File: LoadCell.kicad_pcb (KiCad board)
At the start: 2 copper layers, 51.1 x 38.1 mm, 83 parts, among them J1 M20-8760242, J10 M20-8760242, J11 0.100_1X4, J12 0.100_1X4, J13 M20-8760242, J14 M20-8760242, J15 0.100_1X4, J16 0.100_1X4, J2 M20-8760242, J3 0.100_1X4, J4 0.100_1X4, J5 M20-8760242, J6 M20-8760242, J7 0.100_1X4, J8 0.100_1X4, J9 M20-8760242, U1 MCP6002, U2 MCP6002, U3 MCP6002, U4 MCP6002, U5 MCP6002, U6 MCP6002, U7 MCP6002, U8 MCP6002

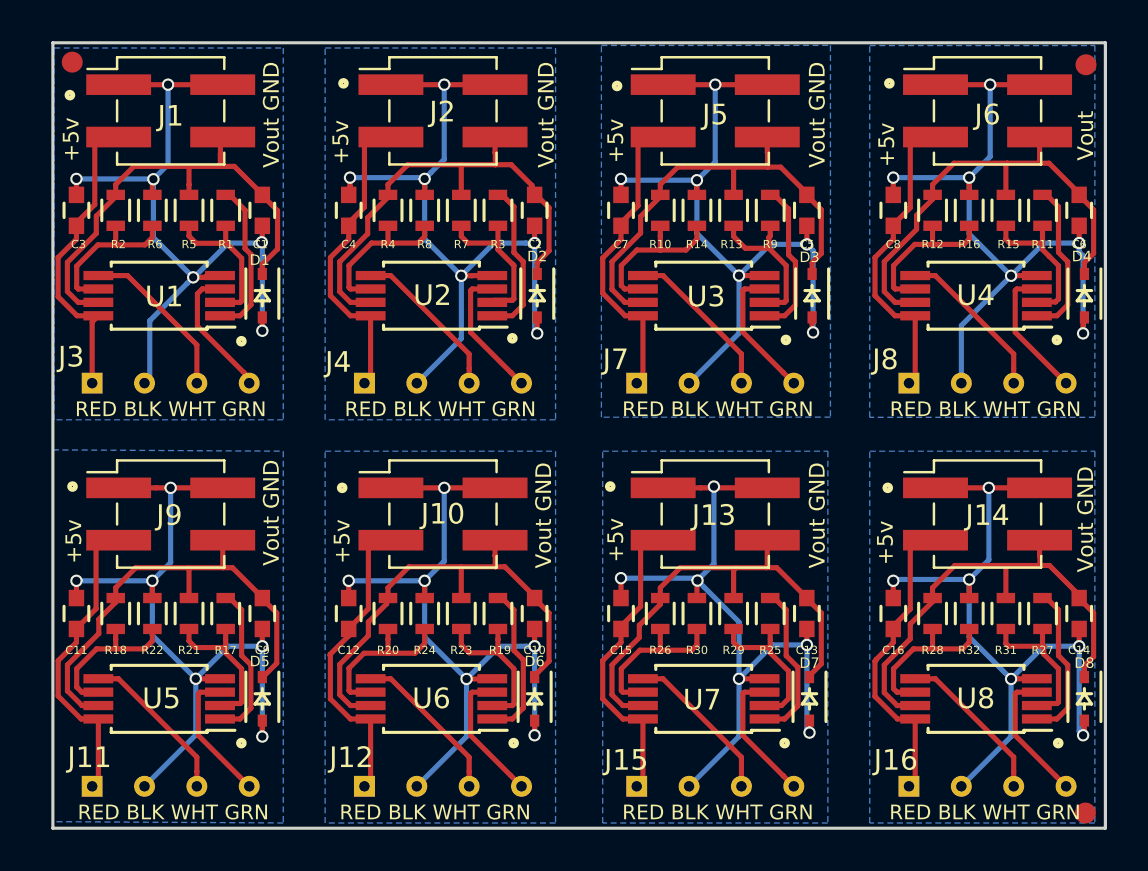
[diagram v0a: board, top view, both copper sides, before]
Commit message: First cut
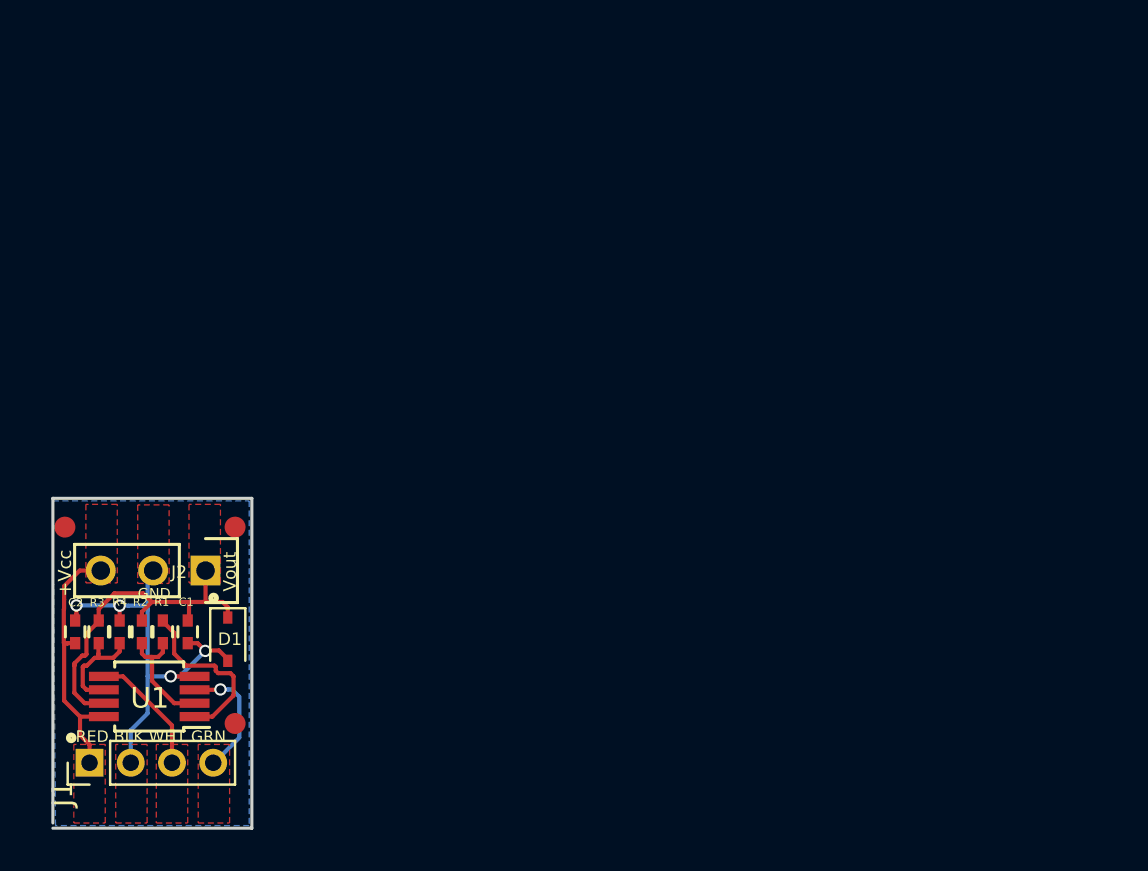
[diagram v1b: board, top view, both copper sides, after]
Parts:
- removed C10, C11, C12, C13, C14, C15, C16, C3, C4, C5, C6, C7, C8, C9: 1uF, _Passive:C_0603
- removed D2, D3, D4, D5, D6, D7, D8: MM3Z3V0ST1G, _Passive:SOD-323
- removed J10, J13, J14, J5, J6, J9: M20-8760242, _Connector:Pin_Header_Straight_2x02_Pitch2.54mm_SMD
- removed J11, J12, J15, J16, J3, J4, J7, J8: 0.100_1X4, _Connector:0.100_1x4_micro
- removed R10, R12, R13, R15, R18, R20, R21, R23, R26, R28, R29, R31, R5, R7: 1K, _Passive:R_0603
- removed R11, R14, R16, R17, R19, R22, R24, R25, R27, R30, R32, R6, R8, R9: 390K, _Passive:R_0603
- removed U2, U3, U4, U5, U6, U7, U8: MCP6002, Housings_SSOP:TSSOP-8_4.4x3mm_Pitch0.65mm
- C1, C2: footprint _Passive:C_0603 -> _Passive:C_0402
- D1: footprint _Passive:SOD-323 -> Diodes_SMD:D_SOD-323
- J1: value M20-8760242 -> 0.100_1X4; footprint _Connector:Pin_Header_Straight_2x02_Pitch2.54mm_SMD -> Socket_Strips:Socket_Strip_Straight_1x04_Pitch2.00mm
- J2: value M20-8760242 -> 22-27-2031; footprint _Connector:Pin_Header_Straight_2x02_Pitch2.54mm_SMD -> _Connector:0.100_1x3_small
- R1, R2: footprint _Passive:R_0603 -> _Passive:R_0402
- R3: value 390K -> 1K; footprint _Passive:R_0603 -> _Passive:R_0402
- R4: value 1K -> 390K; footprint _Passive:R_0603 -> _Passive:R_0402
- U1: value MCP6002 -> LMV358; footprint Housings_SSOP:TSSOP-8_4.4x3mm_Pitch0.65mm -> Housings_SSOP:MSOP-8_3x3mm_Pitch0.65mm
- moved FID2 52.2 mm to (110.4, 96.5)
- moved FID3 43.5 mm to (110.4, 87.0)
- moved J1 31.9 mm to (103.4, 98.4), turned to 90 degrees
- moved C2 30.2 mm to (102.7, 92.1), turned to 90 degrees
- moved R3 28.2 mm to (103.8, 92.1)
- moved J2 26.4 mm to (106.5, 89.1), turned to 270 degrees
- moved R4 24.2 mm to (104.8, 92.1), turned to 270 degrees
- moved FID1 22.6 mm to (102.2, 87.0)
- moved C1 20.8 mm to (108.1, 92.1)
- moved R1 20.7 mm to (106.9, 92.1)
- moved R2 20.5 mm to (105.9, 92.1), turned to 270 degrees
- moved U1 19.4 mm to (106.3, 95.2)
- moved D1 16.7 mm to (110.1, 92.4)
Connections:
- C1 pad 2: /Main Sheet/BLK -> GNDA
- C2 pad 1: Net-(C2-Pad1) -> /Main Sheet/RED
- C2 pad 2: Net-(C2-Pad2) -> GNDA
- D1 pad 2: /Main Sheet/BLK -> GNDA
- J1 pad 1: /Main Sheet/BLK -> /Main Sheet/RED
- J1 pad 2: /Main Sheet/BLK -> GNDA
- J1 pad 3: /Main Sheet/RED -> /Main Sheet/WHT
- J1 pad 4: /Main Sheet/Vout -> /Main Sheet/GRN
- J2 pad 1: Net-(C2-Pad2) -> /Main Sheet/Vout
- J2 pad 2: Net-(C2-Pad2) -> GNDA
- J2 pad 3: Net-(C4-Pad1) -> /Main Sheet/RED
- R2 pad 1: Net-(R2-Pad1) -> /Main Sheet/Vout
- R2 pad 2: /Main Sheet/Vout -> Net-(R1-Pad1)
- R3 pad 2: Net-(R3-Pad2) -> /Main Sheet/Vout
- R4 pad 1: Net-(R4-Pad1) -> GNDA
- R4 pad 2: Net-(C2-Pad1) -> Net-(R3-Pad1)
- U1 pad 4: /Main Sheet/BLK -> GNDA
- U1 pad 6: Net-(R2-Pad1) -> Net-(R3-Pad1)
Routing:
- net Net-(C2-Pad2): track 38.6 -> 0.00 mm, vias 6 -> 0
- net Net-(C6-Pad2): track 38.5 -> 0.00 mm, vias 6 -> 0
- net Net-(C14-Pad2): track 38.4 -> 0.00 mm, vias 6 -> 0
- net Net-(C11-Pad2): track 38.4 -> 0.00 mm, vias 6 -> 0
- net Net-(C13-Pad2): track 38.3 -> 0.00 mm, vias 6 -> 0
- net Net-(C10-Pad2): track 38.2 -> 0.00 mm, vias 6 -> 0
- net Net-(C5-Pad2): track 38.1 -> 0.00 mm, vias 6 -> 0
- net /Main Sheet/BLK: track 37.3 -> 0.00 mm, vias 6 -> 0
- net Net-(C10-Pad1): track 23.5 -> 0.00 mm
- net Net-(C2-Pad1): track 23.5 -> 0.00 mm
- net Net-(C6-Pad1): track 23.3 -> 0.00 mm
- net Net-(C13-Pad1): track 23.3 -> 0.00 mm
- net Net-(C14-Pad1): track 23.2 -> 0.00 mm
- net Net-(C9-Pad1): track 23.2 -> 0.00 mm
- net Net-(C5-Pad1): track 23.0 -> 0.00 mm
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- added copper zone on F.Cu, net /Main Sheet/GRN
- added copper zone on F.Cu, net /Main Sheet/RED
- added copper zone on F.Cu, net /Main Sheet/Vout
- added copper zone on F.Cu, net /Main Sheet/WHT
- added copper zone on B.Cu, net GNDA
- added copper zone on F.Cu, net GNDA
- removed copper zone on B.Cu, net /Main Sheet/BLK
- removed copper zone on B.Cu, net Net-(C10-Pad2)
- removed copper zone on B.Cu, net Net-(C11-Pad2)
- removed copper zone on B.Cu, net Net-(C13-Pad2)
- removed copper zone on B.Cu, net Net-(C14-Pad2)
- removed copper zone on B.Cu, net Net-(C2-Pad2)
- removed copper zone on B.Cu, net Net-(C5-Pad2)
- removed copper zone on B.Cu, net Net-(C6-Pad2)
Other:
- board size 51.1 x 38.1 mm -> 9.7 x 16 mm
- net class Default: clearance 0.2 -> 0.19812; trace_width 0.25 -> 0.2032
- rule trace_clearance: 0.2 -> 0.19812
- rule trace_min: 0.20066 -> 0.2032
- board text added: "+Vcc"
- board text added: "GND"
- board text removed: "+5v"
- board text removed: "Vout GND"
